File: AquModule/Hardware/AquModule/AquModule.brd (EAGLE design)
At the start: 160 x 100 mm, 4 parts

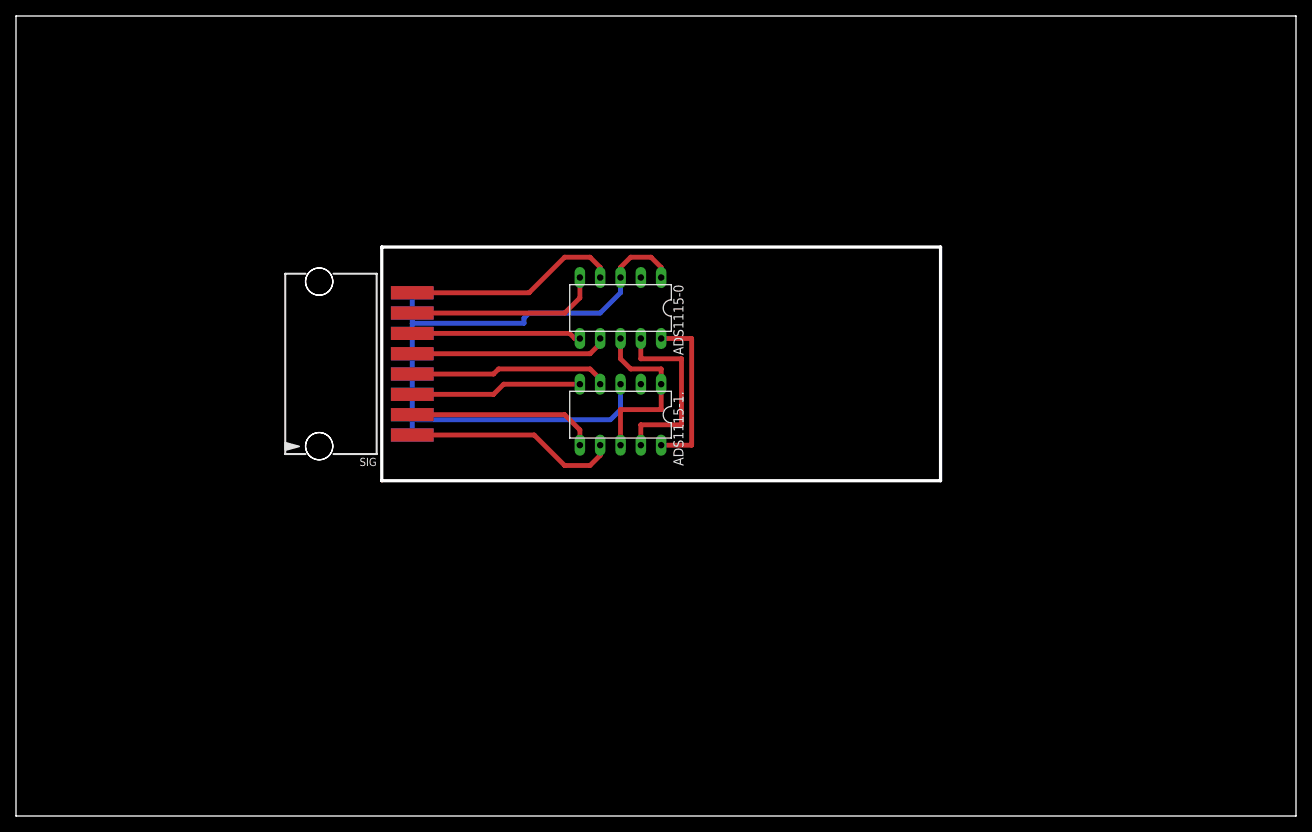
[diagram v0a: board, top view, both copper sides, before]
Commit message: PCB design for module 1 - Ready
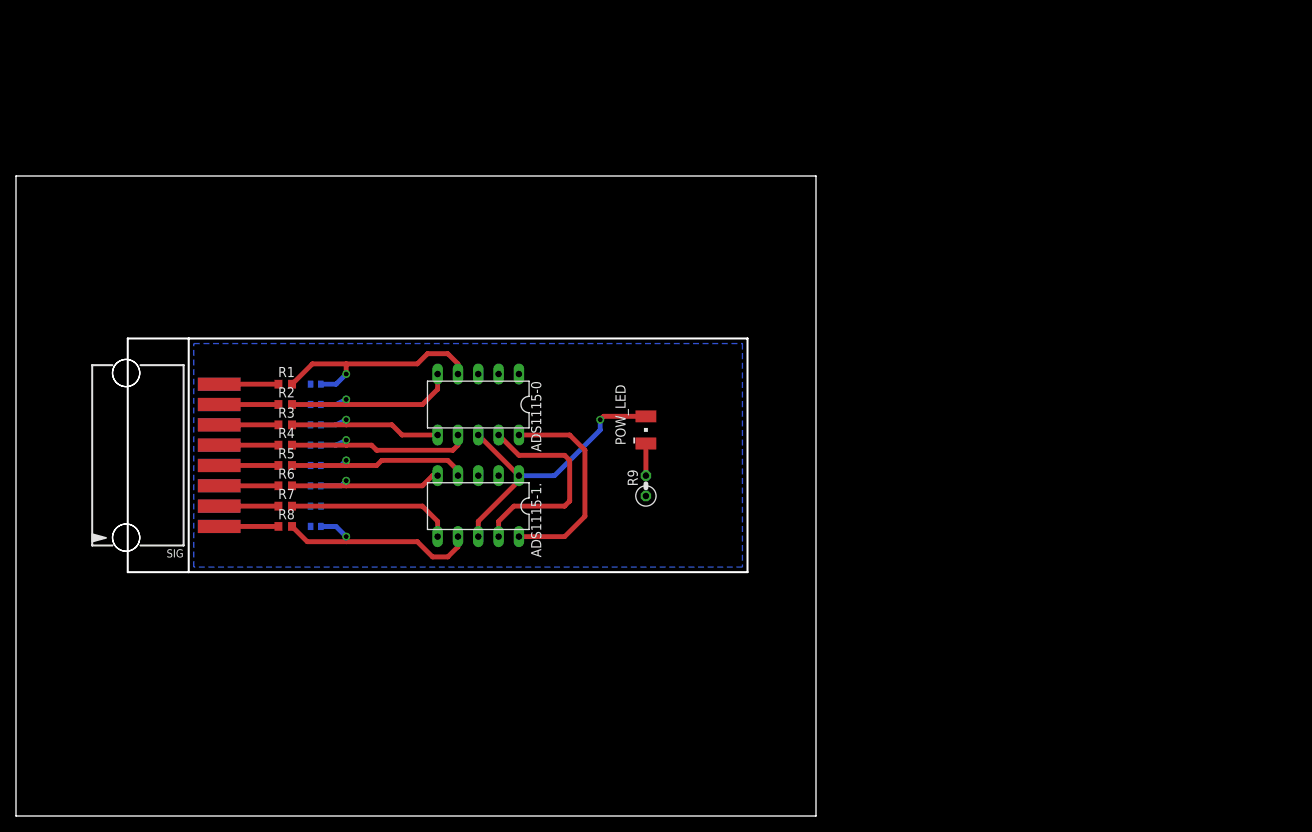
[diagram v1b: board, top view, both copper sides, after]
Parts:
- added C1, C2, C3, C4, C5, C6, C7, C8: 100nF, rcl:C1005
- added POW_LED: LS_T679-D2E2-1, led:PLCC2
- added R1, R2, R3, R4, R5, R6, R7, R8: 1K, resistor:R0603
- added R9: ?, resistor:0207/2V
- moved GND 26.7 mm to (14.6, 45.1)
- moved SIG 26.7 mm to (14.6, 45.1)
- moved ADS1115-0 21.5 mm to (57.8, 51.4)
- moved ADS1115-1. 21.1 mm to (57.8, 38.7)
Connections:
- new net N$10: R2.1, SIG.7
- new net N$11: R3.1, SIG.6
- new net N$12: R4.1, SIG.5
- new net N$13: R5.1, SIG.4
- new net N$14: R6.1, SIG.3
- new net N$15: R7.1, SIG.2
- new net N$16: R8.1, SIG.1
- new net N$17: POW_LED.C, R9.2
- new net N$9: R1.1, SIG.8
- net GND: now also C1.1, C2.1, C3.1, C4.1, C5.1, C6.1, C7.1, C8.1, R9.1
- net N$1: now also C8.2, R1.2; no longer SIG.8
- net N$2: now also C7.2, R2.2; no longer SIG.7
- net N$3: now also C6.2, R3.2; no longer SIG.6
- net N$4: now also C5.2, R4.2; no longer SIG.5
- net N$5: now also C4.2, R5.2; no longer SIG.4
- net N$6: now also C3.2, R6.2; no longer SIG.3
- net N$7: now also C2.2, R7.2; no longer SIG.2
- net N$8: now also C1.2, R8.2; no longer SIG.1
- net VCC: now also POW_LED.A
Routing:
- net GND: track 86.3 -> 0.00 mm
- net VCC: track 22.8 -> 36.6 mm, vias 0 -> 1
- net N$9: track 0.00 -> 7.41 mm
- net N$16: track 0.00 -> 7.41 mm
- net N$15: track 0.00 -> 7.41 mm
- net N$14: track 0.00 -> 7.41 mm
- net N$13: track 0.00 -> 7.41 mm
- net N$12: track 0.00 -> 7.41 mm
- net N$11: track 0.00 -> 7.41 mm
- net N$10: track 0.00 -> 7.41 mm
- net SCL: track 21.0 -> 26.6 mm
- net N$17: track 0.00 -> 4.02 mm
- net SDA: track 23.5 -> 27.1 mm
- net N$7: track 23.6 -> 20.9 mm
- net N$1: track 27.1 -> 29.1 mm, vias 0 -> 1
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- added copper zone on layer 16, net GND
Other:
- board size 160 x 100 mm -> 100 x 80 mm
